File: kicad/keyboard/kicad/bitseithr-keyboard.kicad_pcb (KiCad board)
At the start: 2 copper layers, 365 x 206 mm, 103 parts, among them P2 KEYB CONN 1

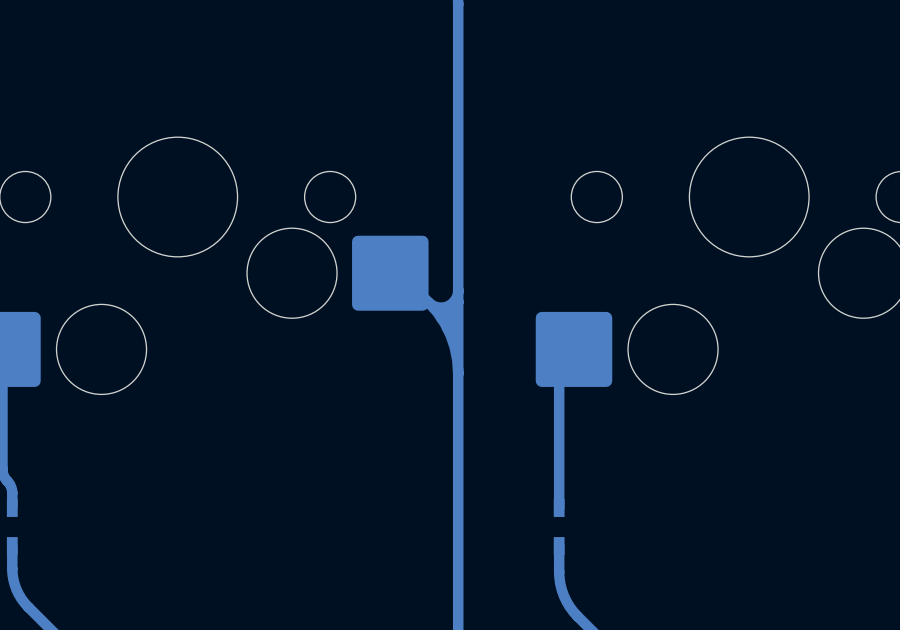
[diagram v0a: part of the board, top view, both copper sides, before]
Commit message: fixed drc warning
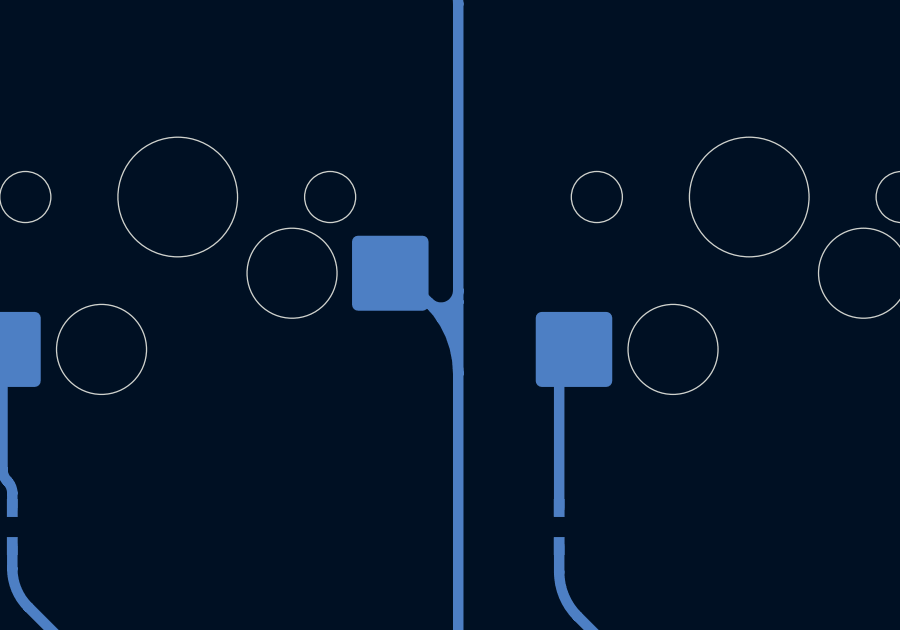
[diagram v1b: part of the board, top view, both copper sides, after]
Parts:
- HOLE (x17): footprint MountingHole:MountingHole_3.5mm -> clholm-kicad-library:MountingHole_M3_GND_7mm
- HOLE (x12): footprint MountingHole:MountingHole_5.7mm -> clholm-kicad-library:MountingHole_5.7mm
